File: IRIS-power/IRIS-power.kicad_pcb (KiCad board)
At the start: 2 copper layers, 66.9 x 65 mm, 83 parts, among them J11 Powerpole, J12 PJ-047AH, J13 IRIS_power_board, Q21 2N7002, Q61 IRLML6402, U11 TVS1400DRV, U12 TVS1400DRV, U21 MAX17261, U31 TPS2121, U41 TPS55340, U51 TPSM53604, U61 LTC3110, U62 PCA9537, U71 TLV75733PDBV

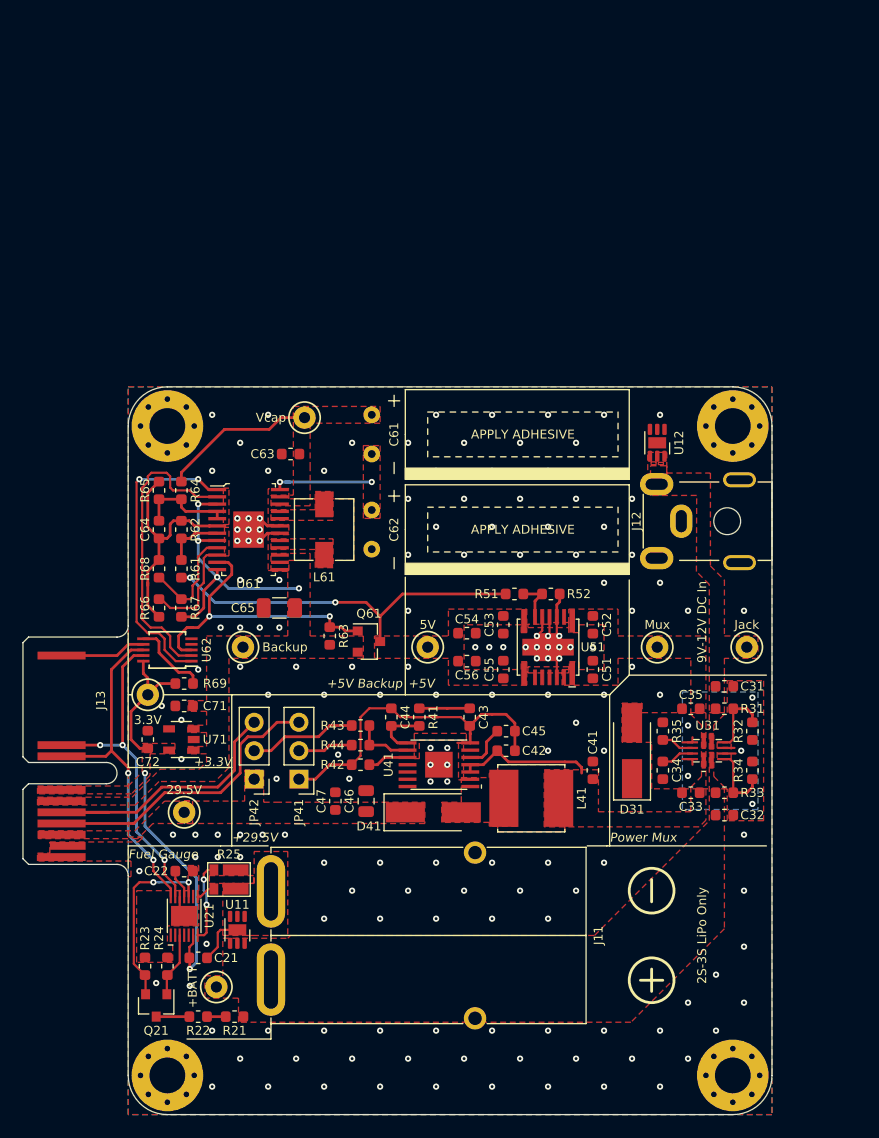
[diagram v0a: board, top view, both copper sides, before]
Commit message: Begin revising for IRIS V4
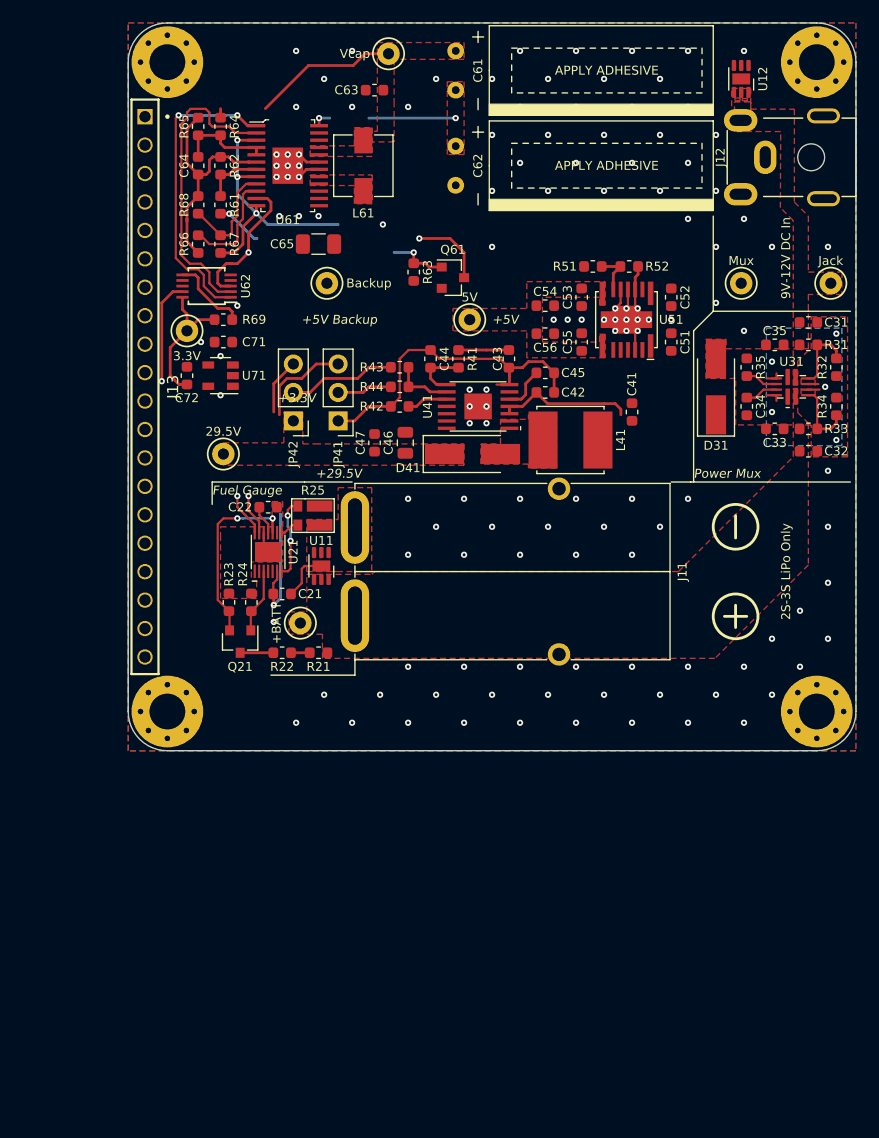
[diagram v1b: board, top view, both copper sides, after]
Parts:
- J13: value IRIS_power_board -> Conn_01x20_MountingPin; footprint star-common-lib:IRIS_Power_Physical -> star-common-lib:IRIS_Muons_physical
- moved C21 33.4 mm to (13.8, 18.5)
- moved C22 33.4 mm to (12.5, 10.8)
- moved C31 33.4 mm to (60.8, -5.75)
- moved C32 33.4 mm to (60.8, 5.75)
- moved C33 33.4 mm to (57.8, 3.75)
- moved C34 33.4 mm to (55.2, 1.75)
- moved C35 33.4 mm to (57.8, -3.75)
- moved C61 33.4 mm to (29.2, -28.2)
- moved C62 33.4 mm to (29.2, -19.8)
- moved C63 33.4 mm to (22.0, -26.5)
- moved D31 33.4 mm to (52.5, 0.00)
- moved J11 33.4 mm to (20.2, 16.5)
- moved J12 33.4 mm to (59.2, -20.5)
- moved Q21 33.4 mm to (10.0, 22.8)
- moved Q61 33.4 mm to (29.0, -9.75)
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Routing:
- net /5V Backup/SCL: track 30.7 -> 3.92 mm, vias 2 -> 1
- net /5V Backup/+5V: track 33.5 -> 10.9 mm
- net /Edge Connector/FB_HV_P: track 26.2 -> 5.01 mm
- net /Edge Connector/FB_HV_N: track 25.7 -> 7.88 mm
- net /5V Backup/SDA: track 30.8 -> 13.5 mm, vias 3 -> 2
- net /3V Supply/+3.3V: track 35.4 -> 24.1 mm, vias 2 -> 1
- net /5V Backup/~CHRG: track 27.6 -> 18.6 mm
- net /5V Backup/~INT: track 7.71 -> 0.00 mm
- net /HV Supply/AGND: track 29.8 -> 28.9 mm
- net GND: vias 163 -> 128
- removed copper zone on F.Cu, net /3V Supply/+3.3V
- removed copper zone on F.Cu, net /3V Supply/VSYS
- removed copper zone on F.Cu, net /5V Supply/+MUX
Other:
- board size 66.9 x 65 mm -> 65 x 65 mm
